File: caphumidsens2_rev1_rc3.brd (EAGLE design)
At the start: 110 x 10 mm, 12 parts, among them IC1 ATtiny25/45/85/13A

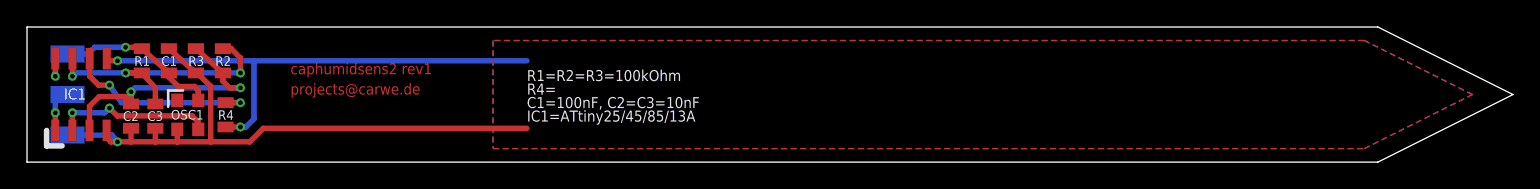
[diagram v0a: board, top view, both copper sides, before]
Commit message: 'improved' routing
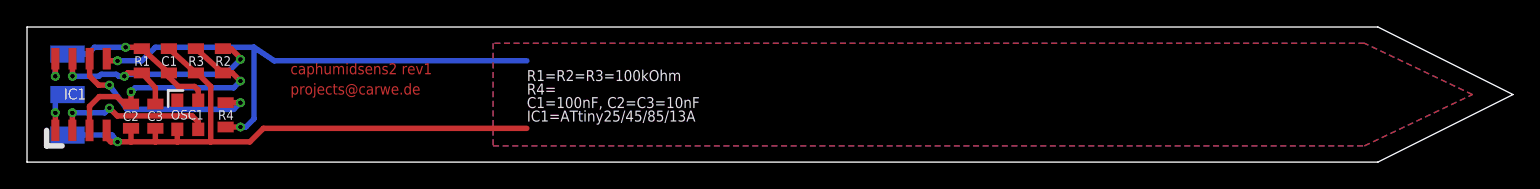
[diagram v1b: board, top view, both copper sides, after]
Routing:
- net SENSE_CAP: track 37.9 -> 39.6 mm
- net 1_3RD_VCC_VREF: track 20.1 -> 19.4 mm
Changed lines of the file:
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@@
 <wire x1="2.095" y1="7.654" x2="2.095" y2="6.35" width="0.4064" layer="1"/>
 <via x="2.095" y="6.35" extent="1-16" drill="0.3302"/>
-<wire x1="8.5" y1="8.4" x2="7.9" y2="8.5" width="0.4064" layer="1"/>
-<wire x1="7.9" y1="8.5" x2="7.3" y2="8.5" width="0.4064" layer="1"/>
+<wire x1="8.5" y1="8.4" x2="8.4" y2="8.5" width="0.4064" layer="1"/>
+<wire x1="8.4" y1="8.5" x2="7.3" y2="8.5" width="0.4064" layer="1"/>
 <via x="7.3" y="8.5" extent="1-16" drill="0.3302"/>
 <contactref element="OSC1" pad="4"/>
@@
 <wire x1="12.675" y1="5.325" x2="12.4" y2="5.6" width="0.4064" layer="1"/>
 <wire x1="12.4" y1="5.6" x2="11.2" y2="5.6" width="0.4064" layer="1"/>
-<wire x1="10.4" y1="6.6" x2="10.5" y2="6.6" width="0.4064" layer="1"/>
 <wire x1="10.5" y1="6.6" x2="10.5" y2="6.3" width="0.4064" layer="1"/>
 <wire x1="10.5" y1="6.3" x2="11.2" y2="5.6" width="0.4064" layer="1"/>
@@
 <contactref element="C1" pad="1"/>
 <polygon width="0.4064" layer="1">
-<vertex x="34.5" y="9"/>
-<vertex x="34.5" y="1"/>
-<vertex x="99" y="1"/>
+<vertex x="34.5" y="8.8"/>
+<vertex x="34.5" y="1.2"/>
+<vertex x="99" y="1.2"/>
 <vertex x="107" y="5"/>
-<vertex x="99" y="9"/>
+<vertex x="99" y="8.8"/>
 </polygon>
 <contactref element="OSC1" pad="2"/>
@@
 <via x="3.365" y="6.35" extent="1-16" drill="0.3302"/>
 <contactref element="C3" pad="2"/>
-<wire x1="9.5" y1="4.5" x2="9.5" y2="4.3" width="0.4064" layer="1"/>
-<wire x1="7.3" y1="6.6" x2="15.8" y2="6.6" width="0.4064" layer="16"/>
-<via x="15.8" y="6.6" extent="1-16" drill="0.3302"/>
-<via x="7.3" y="6.6" extent="1-16" drill="0.3302"/>
-<wire x1="7.3" y1="6.6" x2="8.5" y2="6.6" width="0.4064" layer="1"/>
-<wire x1="3.365" y1="6.35" x2="3.615" y2="6.6" width="0.4064" layer="16"/>
-<wire x1="3.615" y1="6.6" x2="7.3" y2="6.6" width="0.4064" layer="16"/>
+<via x="15.8" y="7.6" extent="1-16" drill="0.3302"/>
 <wire x1="14.5" y1="8.4" x2="15.1" y2="8.4" width="0.4064" layer="1"/>
 <wire x1="15.1" y1="8.4" x2="15.8" y2="7.7" width="0.4064" layer="1"/>
-<wire x1="15.8" y1="7.7" x2="15.8" y2="6.6" width="0.4064" layer="1"/>
+<wire x1="15.8" y1="7.7" x2="15.8" y2="7.6" width="0.4064" layer="1"/>
 <wire x1="8.5" y1="6.6" x2="9.5" y2="5.5" width="0.4064" layer="1"/>
 <wire x1="9.5" y1="5.5" x2="9.5" y2="4.3" width="0.4064" layer="1"/>
+<wire x1="5.5" y1="6.5" x2="5.3" y2="6.35" width="0.4064" layer="16"/>
+<wire x1="5.3" y1="6.35" x2="3.365" y2="6.35" width="0.4064" layer="16"/>
+<wire x1="15.8" y1="7.6" x2="14.7" y2="6.5" width="0.4064" layer="16"/>
+<wire x1="5.5" y1="6.5" x2="6.6" y2="6.5" width="0.4064" layer="16"/>
+<wire x1="6.6" y1="6.5" x2="6.8" y2="6.35" width="0.4064" layer="16"/>
+<wire x1="6.8" y1="6.35" x2="7.2" y2="6.35" width="0.4064" layer="16"/>
+<via x="7.2" y="6.35" extent="1-16" drill="0.3302"/>
+<wire x1="7.2" y1="6.35" x2="7.45" y2="6.6" width="0.4064" layer="1"/>
+<wire x1="7.45" y1="6.6" x2="8.5" y2="6.6" width="0.4064" layer="1"/>
+<wire x1="7.2" y1="6.35" x2="7.35" y2="6.5" width="0.4064" layer="16"/>
+<wire x1="7.35" y1="6.5" x2="14.7" y2="6.5" width="0.4064" layer="16"/>
 </signal>
 <signal name="1_3RD_VCC_VREF">
@@
 <contactref element="C2" pad="1"/>
 <wire x1="4.625" y1="2.346" x2="4.625" y2="4.125" width="0.4064" layer="1"/>
-<via x="15.8" y="5.5" extent="1-16" drill="0.3302"/>
 <via x="7.7" y="5.2" extent="1-16" drill="0.3302"/>
 <wire x1="4.625" y1="4.125" x2="5.35" y2="4.85" width="0.4064" layer="1"/>
-<wire x1="14.5" y1="6.6" x2="14.5" y2="6" width="0.4064" layer="1"/>
-<wire x1="14.5" y1="6" x2="15" y2="5.5" width="0.4064" layer="1"/>
-<wire x1="15" y1="5.5" x2="15.8" y2="5.5" width="0.4064" layer="1"/>
 <wire x1="7.7" y1="5.2" x2="8" y2="5.5" width="0.4064" layer="16"/>
-<wire x1="8" y1="5.5" x2="15.8" y2="5.5" width="0.4064" layer="16"/>
+<wire x1="8" y1="5.5" x2="15.3" y2="5.5" width="0.4064" layer="16"/>
 <wire x1="7.7" y1="5.2" x2="7.7" y2="4.3" width="0.4064" layer="1"/>
-<wire x1="5.35" y1="4.85" x2="7.7" y2="4.85" width="0.4064" layer="1"/>
-<wire x1="7.7" y1="4.85" x2="7.7" y2="4.3" width="0.4064" layer="1"/>
 <wire x1="12.5" y1="8.4" x2="14.5" y2="6.6" width="0.4064" layer="1"/>
+<wire x1="14.5" y1="6.6" x2="15.2" y2="6.6" width="0.4064" layer="1"/>
+<wire x1="15.2" y1="6.6" x2="15.8" y2="6" width="0.4064" layer="1"/>
+<via x="15.8" y="6" extent="1-16" drill="0.3302"/>
+<wire x1="15.3" y1="5.5" x2="15.8" y2="6" width="0.4064" layer="16"/>
+<wire x1="7.7" y1="4.3" x2="7.2" y2="4.3" width="0.4064" layer="1"/>
+<wire x1="7.2" y1="4.3" x2="6.65" y2="4.85" width="0.4064" layer="1"/>
+<wire x1="6.65" y1="4.85" x2="5.35" y2="4.85" width="0.4064" layer="1"/>
 </signal>
 <signal name="SENSE_CAP">
 <contactref element="IC1" pad="5"/>
 <polygon width="0.4064" layer="16">
-<vertex x="34.5" y="9"/>
-<vertex x="34.5" y="1"/>
-<vertex x="99" y="1"/>
+<vertex x="34.5" y="8.8"/>
+<vertex x="34.5" y="1.2"/>
+<vertex x="99" y="1.2"/>
 <vertex x="107" y="5"/>
-<vertex x="99" y="9"/>
+<vertex x="99" y="8.8"/>
 </polygon>
-<wire x1="6.7" y1="7.5" x2="16.8" y2="7.5" width="0.4064" layer="16"/>
-<wire x1="16.8" y1="7.5" x2="37" y2="7.5" width="0.4064" layer="16"/>
+<wire x1="6.7" y1="7.5" x2="8.5" y2="7.5" width="0.4064" layer="16"/>
+<wire x1="8.5" y1="7.5" x2="9.5" y2="8.5" width="0.4064" layer="16"/>
+<wire x1="9.5" y1="8.5" x2="16.8" y2="8.5" width="0.4064" layer="16"/>
+<wire x1="16.8" y1="8.5" x2="18.3" y2="7.5" width="0.4064" layer="16"/>
+<wire x1="18.3" y1="7.5" x2="37" y2="7.5" width="0.4064" layer="16"/>
 <via x="6.7" y="7.5" extent="1-16" drill="0.3302"/>
 <contactref element="R4" pad="1"/>
-<wire x1="16.8" y1="3.2" x2="16.8" y2="7.5" width="0.4064" layer="16"/>
+<wire x1="16.8" y1="3.2" x2="16.8" y2="8.5" width="0.4064" layer="16"/>
 <wire x1="6.7" y1="7.5" x2="5.905" y2="7.5" width="0.4064" layer="1"/>
 <wire x1="5.905" y1="7.5" x2="5.905" y2="7.654" width="0.4064" layer="1"/>
@@
 <contactref element="IC1" pad="6"/>
 <contactref element="R4" pad="2"/>
-<wire x1="7" y1="4.4" x2="6.1" y2="5.7" width="0.4064" layer="16"/>
+<wire x1="7.4" y1="3.9" x2="6.1" y2="5.7" width="0.4064" layer="16"/>
 <wire x1="14.7" y1="4.4" x2="15.8" y2="4.4" width="0.4064" layer="1"/>
 <via x="15.8" y="4.4" extent="1-16" drill="0.3302"/>
 <via x="6.1" y="5.7" extent="1-16" drill="0.3302"/>
-<wire x1="7" y1="4.4" x2="15.8" y2="4.4" width="0.4064" layer="16"/>
+<wire x1="7.4" y1="3.9" x2="15.3" y2="3.9" width="0.4064" layer="16"/>
+<wire x1="15.3" y1="3.9" x2="15.8" y2="4.4" width="0.4064" layer="16"/>
 <wire x1="4.635" y1="7.654" x2="4.635" y2="6.365" width="0.4064" layer="1"/>
 <wire x1="4.635" y1="6.365" x2="5.3" y2="5.7" width="0.4064" layer="1"/>
